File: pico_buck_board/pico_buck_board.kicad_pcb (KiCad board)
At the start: 2 copper layers, 89.4 x 88.2 mm, 72 parts, among them J101 Conn_01x02, J102 part_of_pico, J103 Conn_01x02, J104 Conn_01x02, J105 Conn_01x02, Q201 KST5551MTF, Q202 FSD4435, Q203 KST5551MTF, Q204 FSD4435, Q301 KST5551MTF, Q302 FSD4435, Q303 KST5551MTF, Q304 FSD4435, Q401 KST5551MTF, Q402 FSD4435, Q403 KST5551MTF, Q404 FSD4435

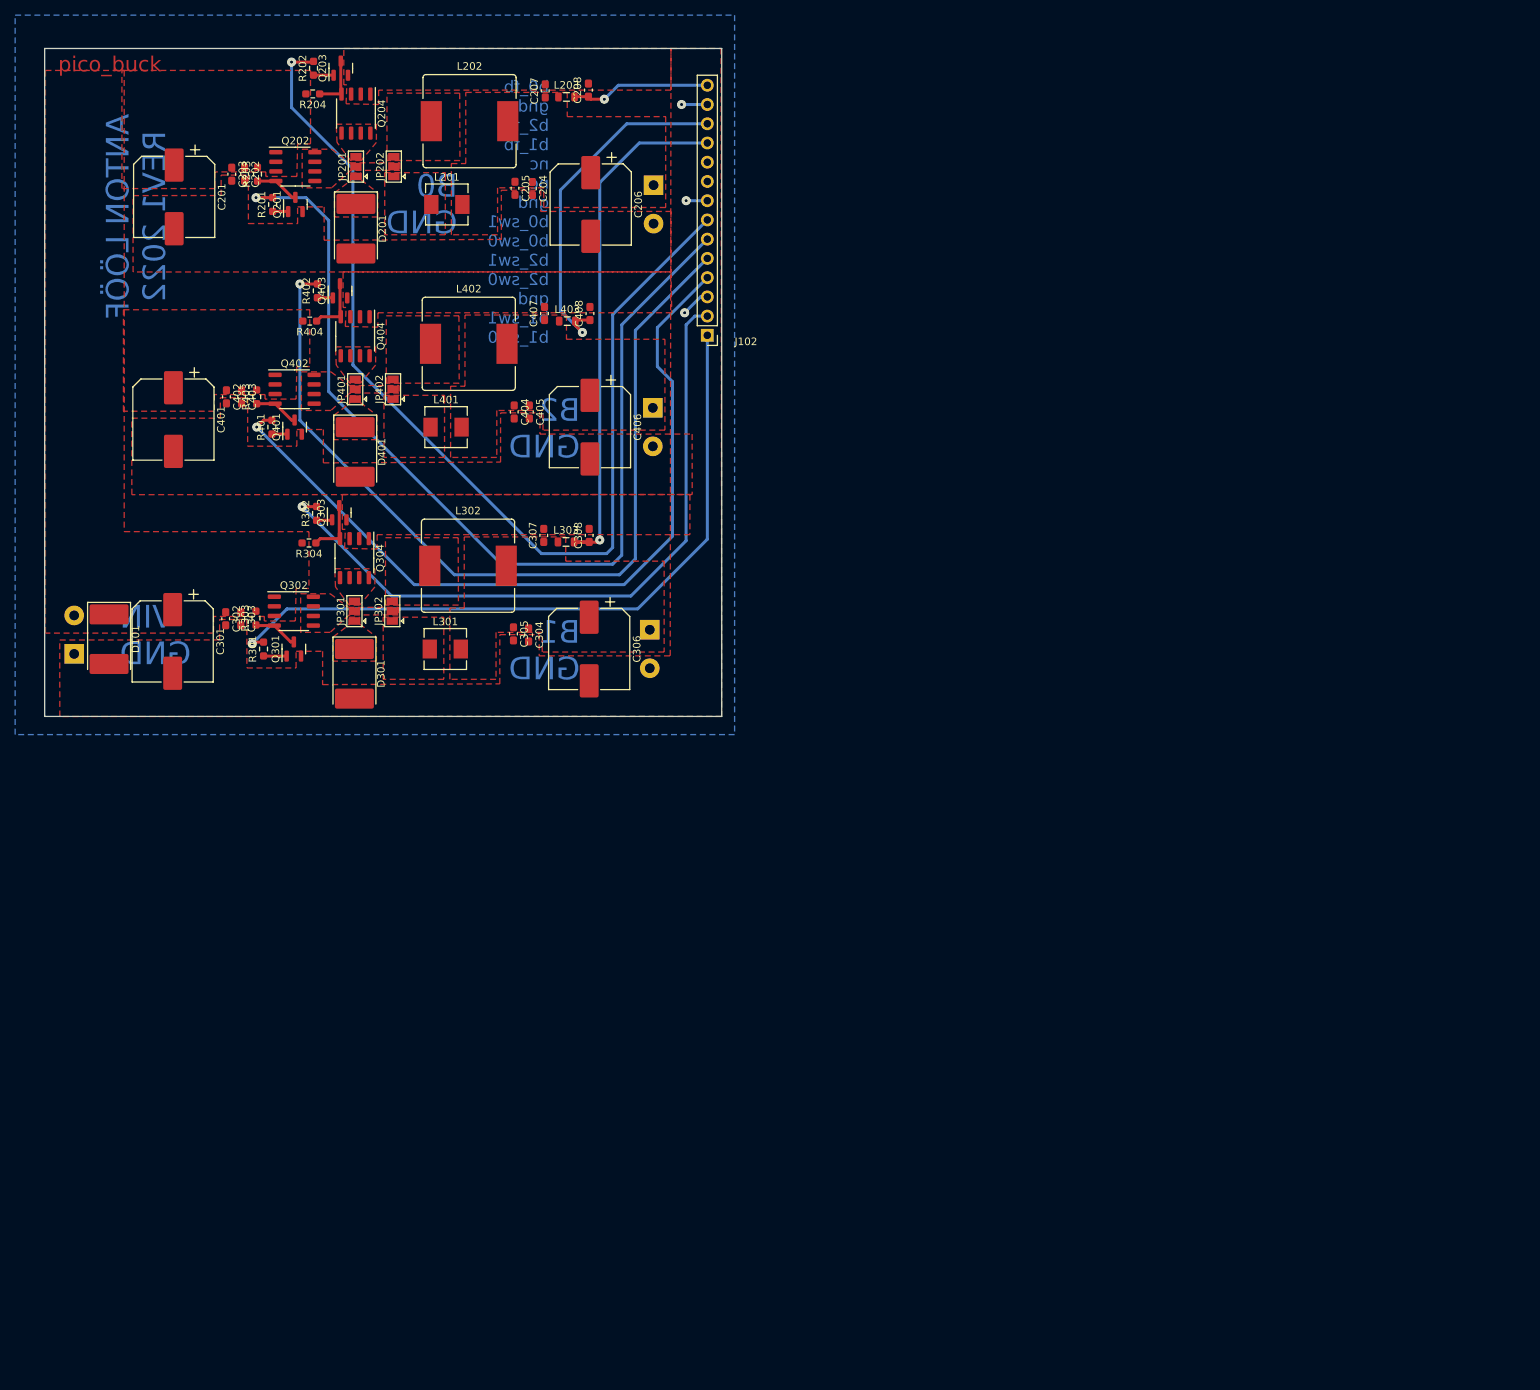
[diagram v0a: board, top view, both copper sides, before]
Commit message: add spwm sw
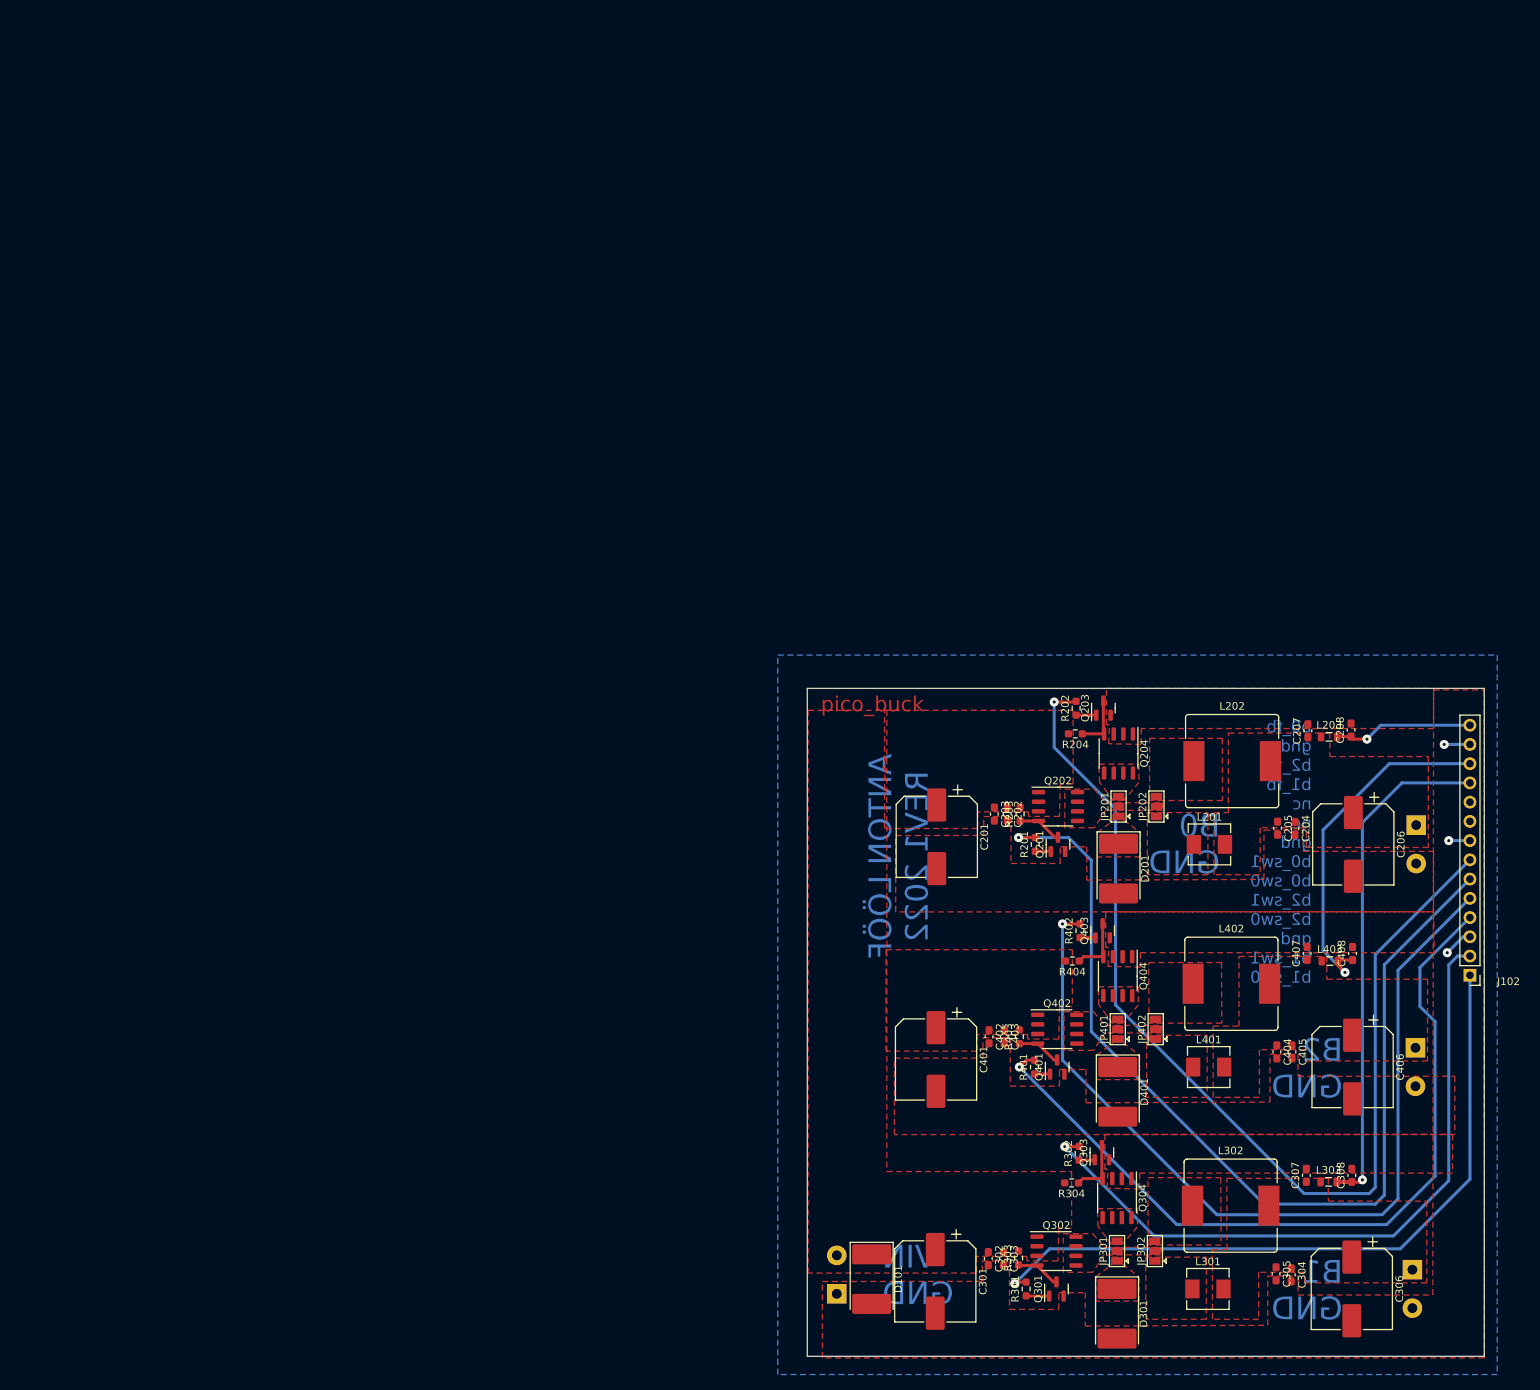
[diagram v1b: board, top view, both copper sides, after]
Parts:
- moved C203 131.5 mm to (204.3, 115.5)
- moved C208 131.5 mm to (251.4, 104.4)
- moved J102 131.5 mm to (267.1, 136.8)
- moved C201 131.5 mm to (196.7, 118.5)
- moved C202 131.5 mm to (206.0, 115.5)
- moved C204 131.5 mm to (244.0, 117.4)
- moved C205 131.5 mm to (241.7, 117.4)
- moved C206 131.5 mm to (251.7, 119.5)
- moved C207 131.5 mm to (245.7, 104.5)
- moved C301 131.5 mm to (196.5, 177.2)
- moved C302 131.5 mm to (203.5, 174.2)
- moved C303 131.5 mm to (205.5, 174.2)
- moved C304 131.5 mm to (243.5, 176.3)
- moved C305 131.5 mm to (241.5, 176.2)
- moved C306 131.5 mm to (251.5, 178.2)
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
